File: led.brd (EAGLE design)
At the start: 14 x 26 mm, 7 parts

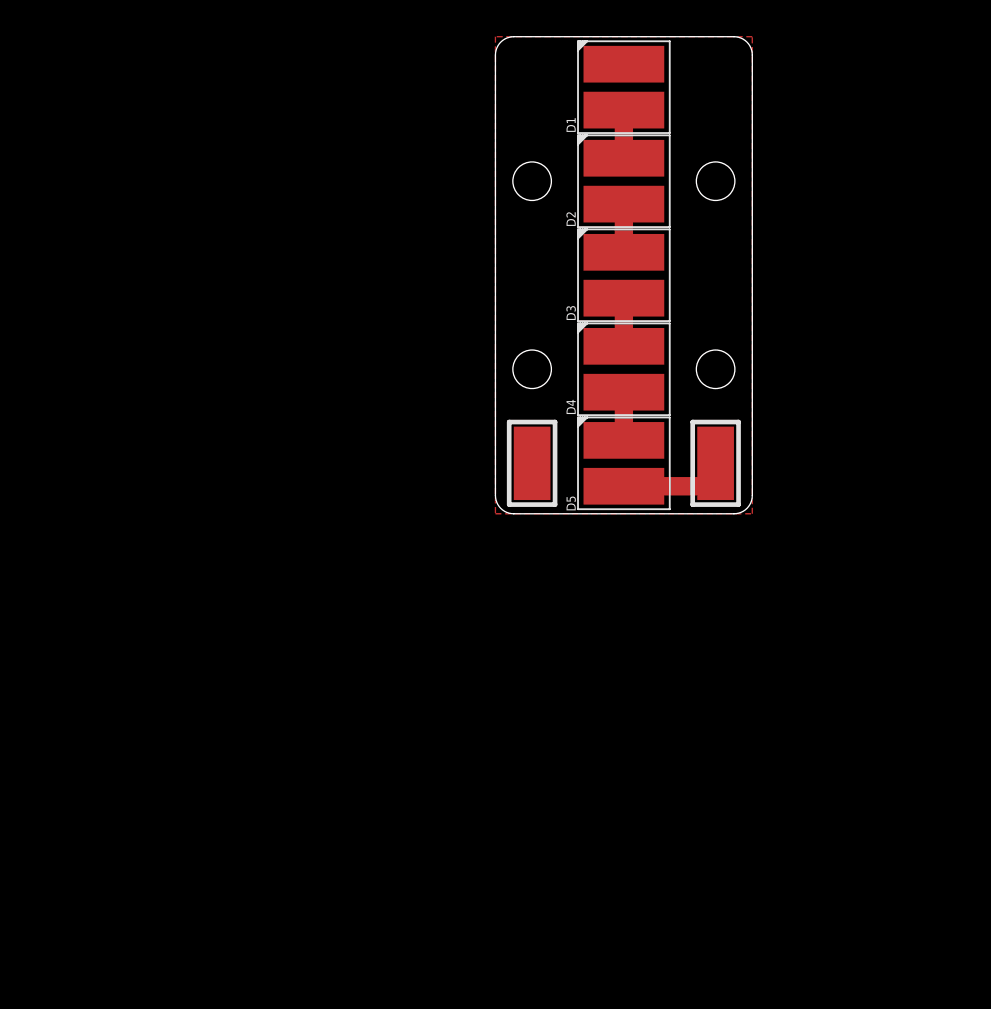
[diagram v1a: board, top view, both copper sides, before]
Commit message: Progress
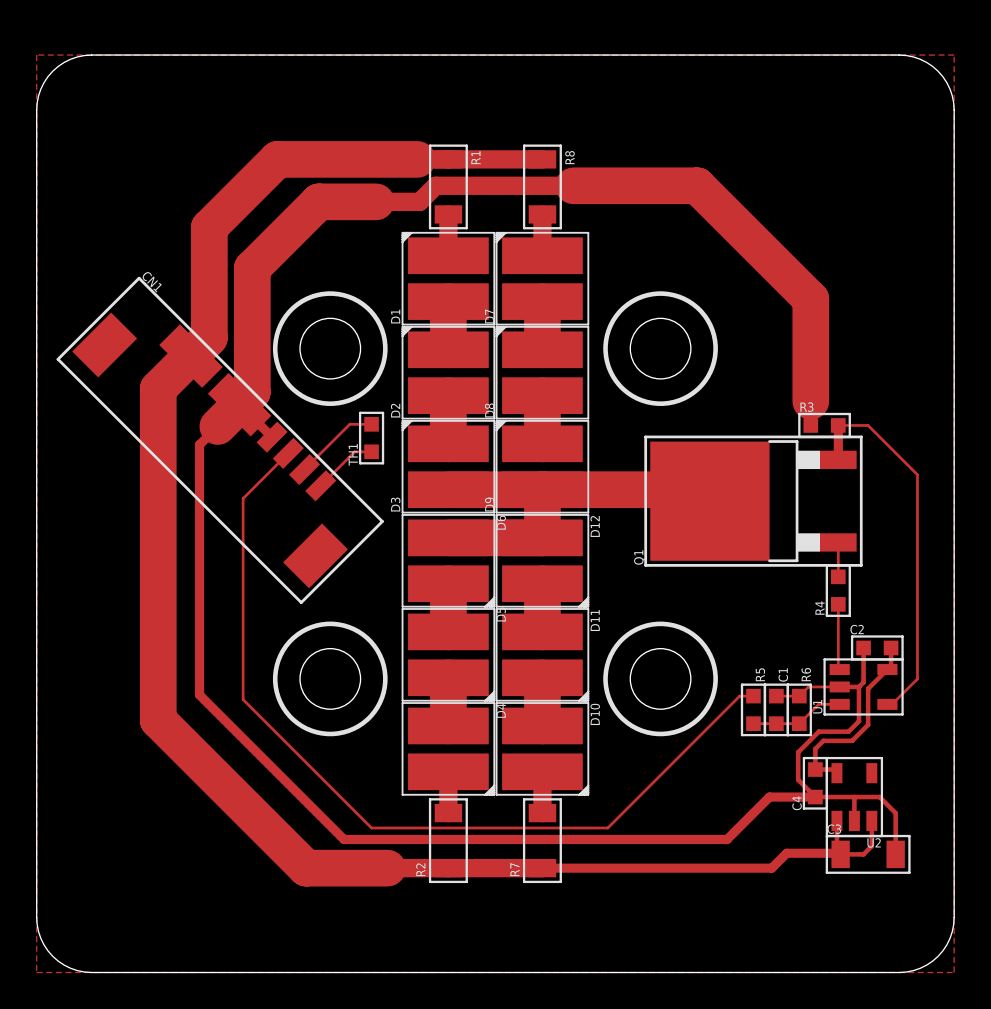
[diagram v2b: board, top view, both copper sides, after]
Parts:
- removed TP1, TP2: TEST_POINT_SQUARE, MISC:OSPREY_HSS_PAD
- added C1, C2: 0.1uF 50V, c_0603:0603
- added C3: 1uF 50V, c_1206:1206
- added C4: 2.2uF 10V, c_0603:0603
- added CN1: JST GH 10 Pin, CONNECTORs:1.25-10PWT
- added D10, D11, D12, D6, D7, D8, D9: 5000K, OPTO:LH502C
- added MECH1, MECH2, MECH3, MECH4: 6mm x 3mm, MISC:MOUNTHOLE_6X3
- added Q1: FDD5612, TRANSISTORs:TO252
- added R1, R2, R7, R8: 1R, RESISTORS:1206
- added R3: 0.33R, RESISTORS:0603
- added R4: 100R, r_0603:0603
- added R5: 20k, r_0603:0603
- added R6: 10k, r_0603:0603
- added TH1: 10k 4037k, RESISTORS:0603
- added U1: NCS20071, ICs:SOT23-5
- added U2: TPS70950, ICs:SOT23-5
- moved D4 22.8 mm to (-2.56, -12.8), turned to 270 degrees
- moved D1 14.2 mm to (-2.56, 12.8)
- moved D2 14.2 mm to (-2.56, 7.69)
- moved D3 14.2 mm to (-2.56, 2.56)
- moved D5 14.2 mm to (-2.56, -7.69), turned to 270 degrees
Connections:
- removed net A: D1.A, TP1.1
- removed net K: D5.K, TP2.1
- new net GND: C1.1, C2.1, C3.1, C4.1, CN1.4, CN1.5, CN1.6, CN1.7, R3.1, R6.1, U1.2, U2.2
- new net LED_PWM_CONT: CN1.8, R5.1
- new net N$10: D11.K, D12.A
- new net N$11: D10.K, D11.A
- new net N$13: D1.A, R1.1
- new net N$16: D12.K, D3.K, D6.K, D9.K, Q1.2
- new net N$17: C1.2, R5.2, R6.2, U1.3
- new net N$18: Q1.1, R4.2
- new net N$19: R4.1, U1.1
- new net N$20: Q1.3, R3.2, U1.4
- new net N$22: C2.2, C4.2, U1.5, U2.5
- new net N$5: D5.K, D6.A
- new net N$6: D4.A, R2.1
- new net N$7: D8.K, D9.A
- new net N$8: D10.A, R7.1
- new net N$9: D7.A, R8.1
- new net PWR_LED_24V: C3.2, CN1.1, CN1.2, CN1.3, R1.2, R2.2, R7.2, R8.2, U2.1, U2.3
- new net TEMP_SEN_A: CN1.9, TH1.2
- new net TEMP_SEN_B: CN1.10, TH1.1
- net N$3: now also D7.K, D8.A; no longer D3.K, D4.A
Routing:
- net GND: track 0.00 -> 131.6 mm
- net PWR_LED_24V: track 0.00 -> 96.2 mm
- net LED_PWM_CONT: track 0.00 -> 48.1 mm
- net N$16: track 0.00 -> 22.3 mm
- net N$20: track 0.00 -> 20.6 mm
- net N$22: track 0.00 -> 10.5 mm
- net K: track 6.03 -> 0.00 mm
- net N$17: track 0.00 -> 5.13 mm
- net TEMP_SEN_A: track 0.00 -> 4.68 mm
- net N$19: track 0.00 -> 3.58 mm
- net TEMP_SEN_B: track 0.00 -> 3.54 mm
- net N$7: track 0.00 -> 2.62 mm
- net N$5: track 0.00 -> 2.62 mm
- net N$11: track 0.00 -> 2.62 mm
- net N$10: track 0.00 -> 2.62 mm
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- added copper zone on layer 1, net PLANE
- removed copper zone on layer 1, net A
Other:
- board size 14 x 26 mm -> 50 x 50 mm
